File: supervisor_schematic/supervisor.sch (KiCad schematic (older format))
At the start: 31 parts, among them J1 Conn_01x08, J16 Conn_01x06_Female, J17 Conn_01x04_Female, J2 Conn_01x05, SW1 SW_Push, SW2 SW_Push, SW3 SW_Push, U1 74HC14, U2 RFM9-LoRa-Radio

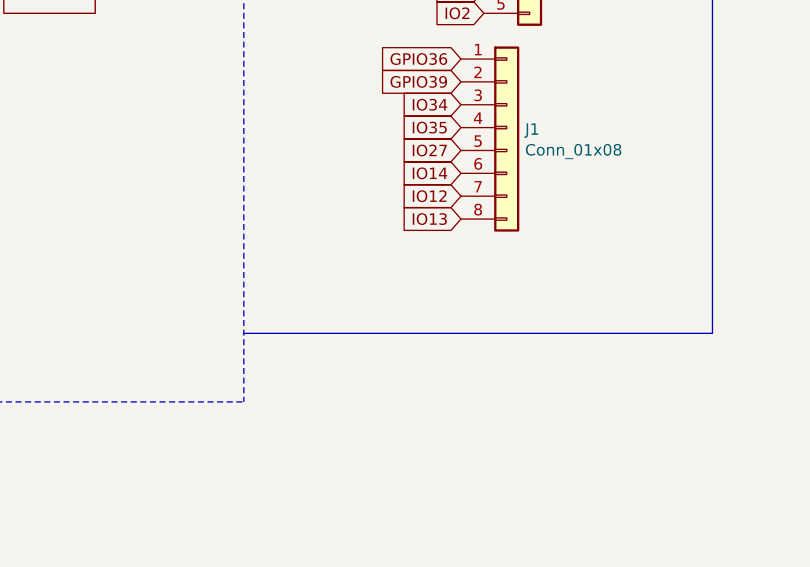
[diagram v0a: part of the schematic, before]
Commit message: supervisor done
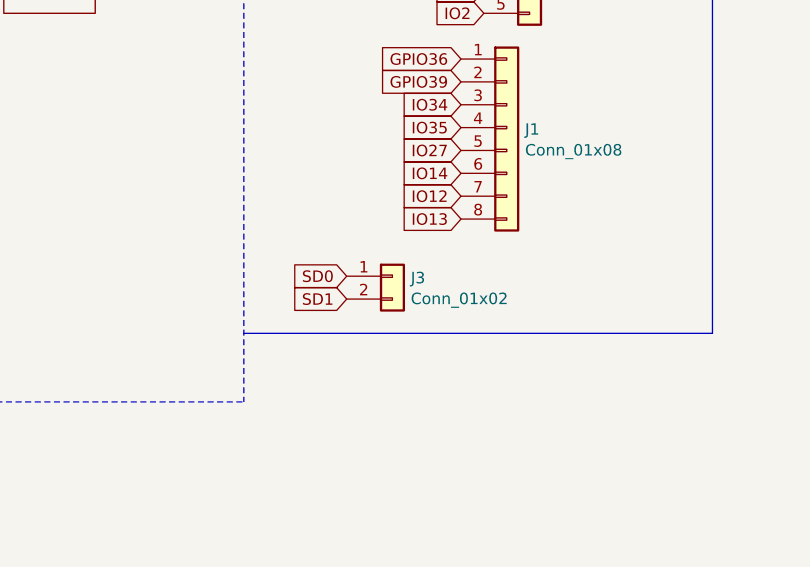
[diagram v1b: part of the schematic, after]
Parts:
- added J3: Conn_01x02, Connector_PinHeader_2.54mm:PinHeader_1x02_P2.54mm_Vertical, symbol Connector_Generic:Conn_01x02
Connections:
- net SD0: now also J3.1 (Pin_1)
- net SD1: now also J3.2 (Pin_2)
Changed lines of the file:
@@
 Wire Wire Line
 	2950 6750 3050 6750
+$Comp
+L Connector_Generic:Conn_01x02 J3
+U 1 1 6232DD59
+P 7000 4150
+F 0 "J3" H 7080 4142 50  0000 L CNN
+F 1 "Conn_01x02" H 7080 4051 50  0000 L CNN
+F 2 "Connector_PinHeader_2.54mm:PinHeader_1x02_P2.54mm_Vertical" H 7000 4150 50  0001 C CNN
+F 3 "~" H 7000 4150 50  0001 C CNN
+	1    7000 4150
+	1    0    0    -1
+$EndComp
+Text GLabel 6800 4150 0    50   Input ~ 0
+SD0
+Text GLabel 6800 4250 0    50   Input ~ 0
+SD1
 $EndSCHEMATC
